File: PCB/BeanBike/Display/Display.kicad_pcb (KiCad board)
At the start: 2 copper layers, 65 x 30 mm, 4 parts, among them J1 Pi 0 2W, J2 Power Conn, J3 Data Conn, J5 Display Conn

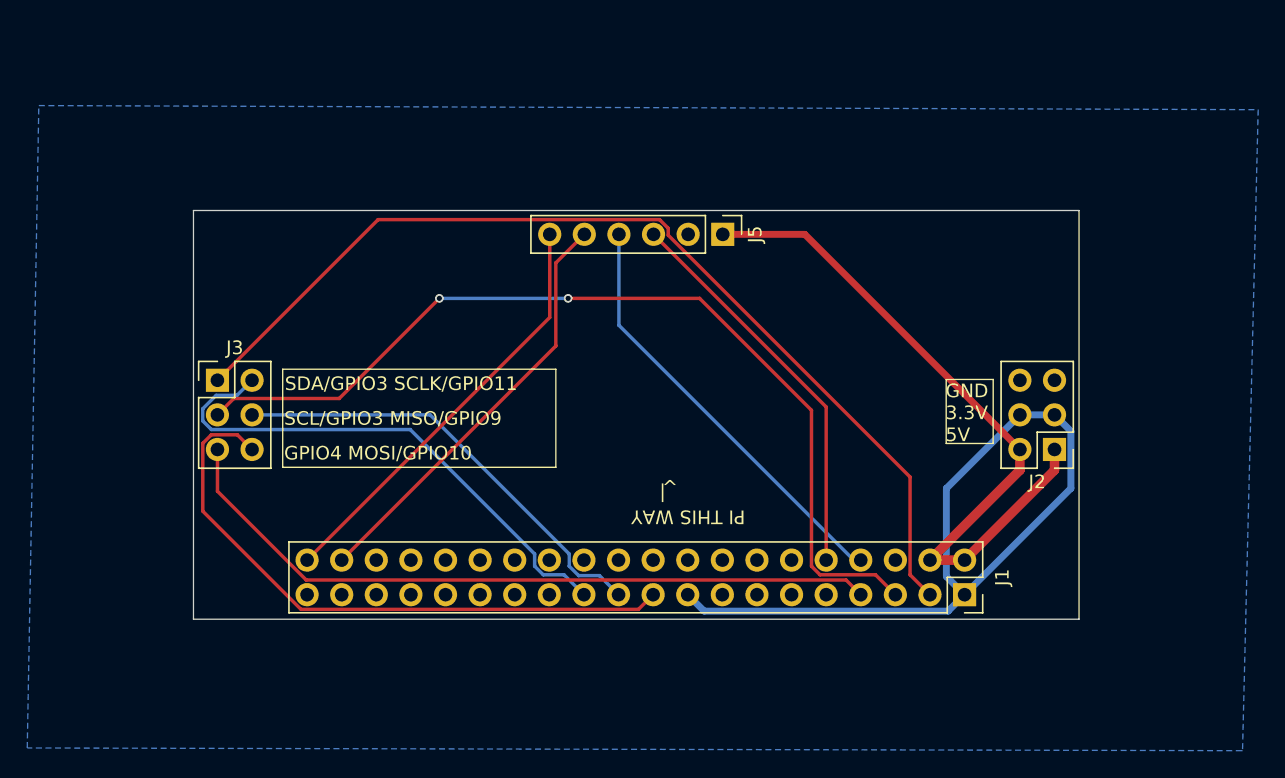
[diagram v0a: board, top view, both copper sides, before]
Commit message: Finish up
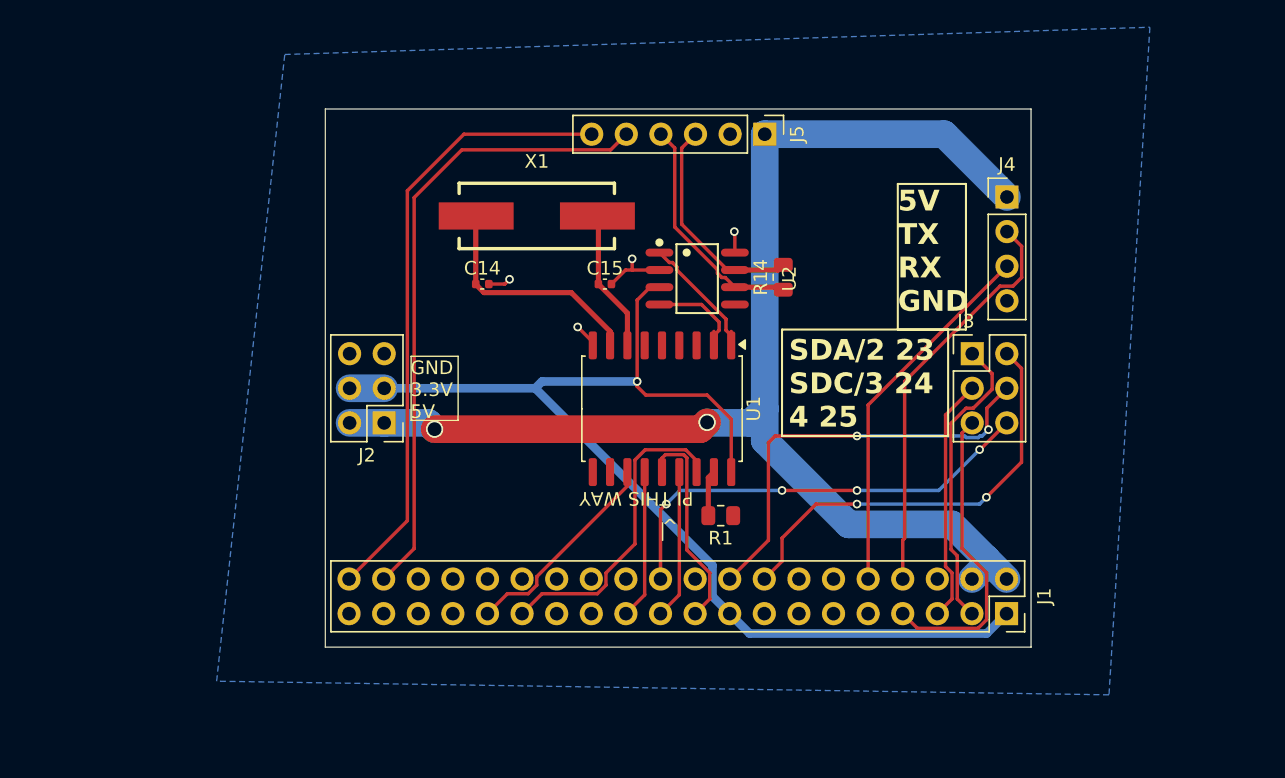
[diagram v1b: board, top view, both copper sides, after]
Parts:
- added C14: 30pF, Capacitor_SMD:C_0402_1005Metric, F.Cu at (156.5, 64.3)
- added C15: 30pF, Capacitor_SMD:C_0402_1005Metric, F.Cu at (165.5, 64.3)
- added J4: GPS/DEBUG, Connector_PinHeader_2.54mm:PinHeader_1x04_P2.54mm_Vertical, F.Cu at (195.0, 58.0)
- added R1: 10k, Resistor_SMD:R_0805_2012Metric, F.Cu at (174.0, 81.3)
- added R14: 120, Resistor_SMD:R_0805_2012Metric, F.Cu at (178.6, 63.9)
- added U1: MCP2515-xSO, Package_SO:SOIC-18W_7.5x11.6mm_P1.27mm, F.Cu at (169.7, 73.5)
- added U2: SN65HVD230DR, easyeda2kicad:SOIC-8_L4.9-W3.9-P1.27-LS6.0-BL, F.Cu at (172.3, 64.0)
- added X1: X49SM8MSD2SC, easyeda2kicad:CRYSTAL-SMD_L11.5-W4.8-LS12.7, F.Cu at (160.5, 59.4)
- moved J3 55.4 mm to (192.5, 69.5)
- moved J2 49.2 mm to (149.3, 74.5)
- moved J5 7.97 mm to (177.2, 53.4)
- moved J1 3.38 mm to (195.0, 88.5)
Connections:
- J1 pad 10: MCU-RX -> PI-RX
- J1 pad 16: unconnected-(J1-Pin_16-Pad16) -> GPIO23
- J1 pad 18: unconnected-(J1-Pin_18-Pad18) -> GPIO24
- J1 pad 22: unconnected-(J1-Pin_22-Pad22) -> GPIO25
- J1 pad 29: unconnected-(J1-Pin_29-Pad29) -> CAN_CS/GPIO5
- J1 pad 31: unconnected-(J1-Pin_31-Pad31) -> CAN_INT/GPIO6
- J1 pad 8: MCU-TX -> PI-TX
- J3 pad 2: SCLK/GPIO11 -> GPIO23
- J3 pad 4: MISO/GPIO9 -> GPIO24
- J3 pad 6: MOSI/GPIO10 -> GPIO25
- J5 pad 3: MCU-RX -> /CAN+
- J5 pad 4: MCU-TX -> /CAN-
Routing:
- net SDA_I2C/GPIO2: track 73.1 -> 21.9 mm
- net SDC_I2c/GPIO3: track 69.0 -> 18.0 mm, vias 2 -> 0
- net +5V: track 52.6 -> 97.4 mm, vias 0 -> 2
- net GPIO25: track 0.00 -> 33.1 mm, vias 0 -> 4
- net GPIO23: track 0.00 -> 31.8 mm, vias 0 -> 2
- net MCU-TX: track 31.6 -> 0.00 mm
- net GPIO24: track 0.00 -> 31.6 mm, vias 0 -> 2
- net GPIO4: track 53.4 -> 22.4 mm
- net MOSI/GPIO10: track 45.8 -> 15.6 mm
- net PI-TX: track 0.00 -> 30.1 mm
- net MCU-RX: track 29.2 -> 0.00 mm
- net +3V3: track 56.8 -> 85.4 mm, vias 0 -> 1
- net SCLK/GPIO11: track 39.2 -> 11.0 mm
- net PI-RX: track 0.00 -> 27.2 mm
- net CAN_CS/GPIO5: track 0.00 -> 23.1 mm
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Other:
- board size 65 x 30 mm -> 51.8 x 39.5 mm
- board text added: "5V TX RX GND"
- board text added: "BeanBike Display"
- board text added: "Giovanni Antenucci"
- board text added: "SDA/2 23 SDC/3 24 4 25"
- board text removed: "BeanBike Display Ginobeano"
- board text removed: "GPIO4 MOSI/GPIO10"
- board text removed: "SCL/GPIO3 MISO/GPIO9"
- board text removed: "SDA/GPIO3 SCLK/GPIO11"
